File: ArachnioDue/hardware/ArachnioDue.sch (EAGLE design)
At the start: 55 parts, among them J6 HEAD17-NOSS, Q1 12MHz, U1 SAM3SB-AU, U2 AP2111HA-3.3

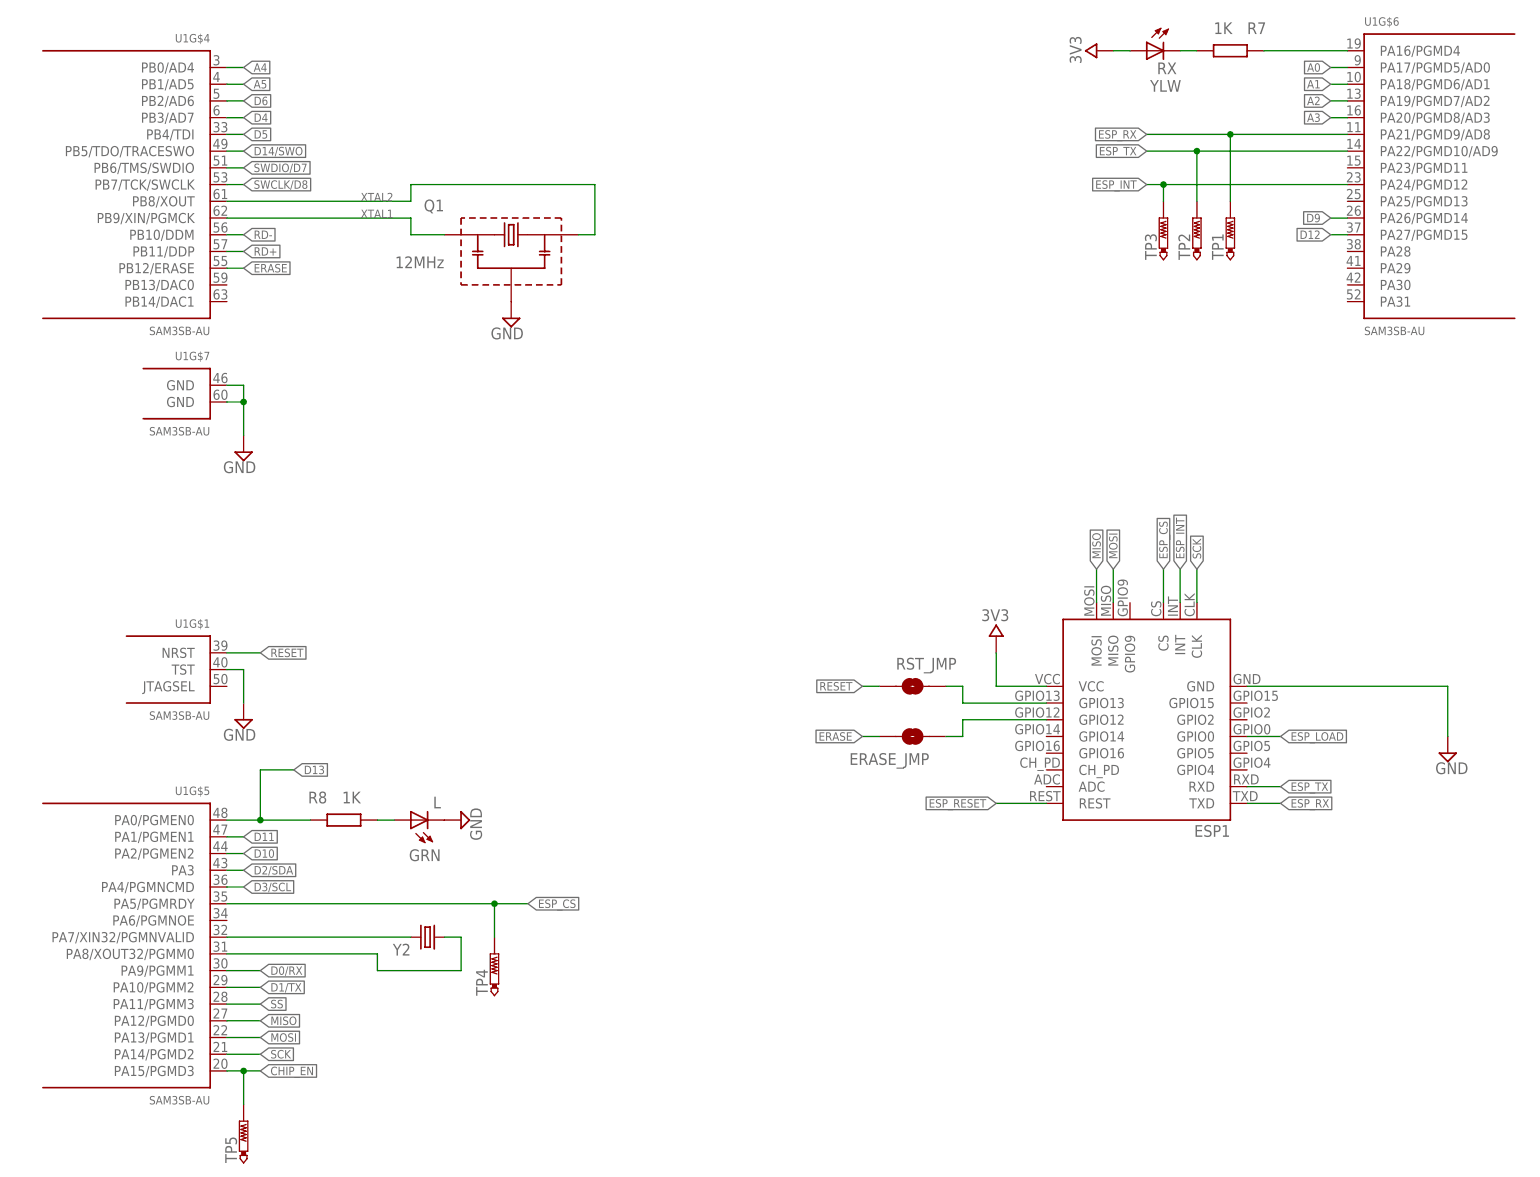
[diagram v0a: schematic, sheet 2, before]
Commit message: Some last changes to the schematic and layout
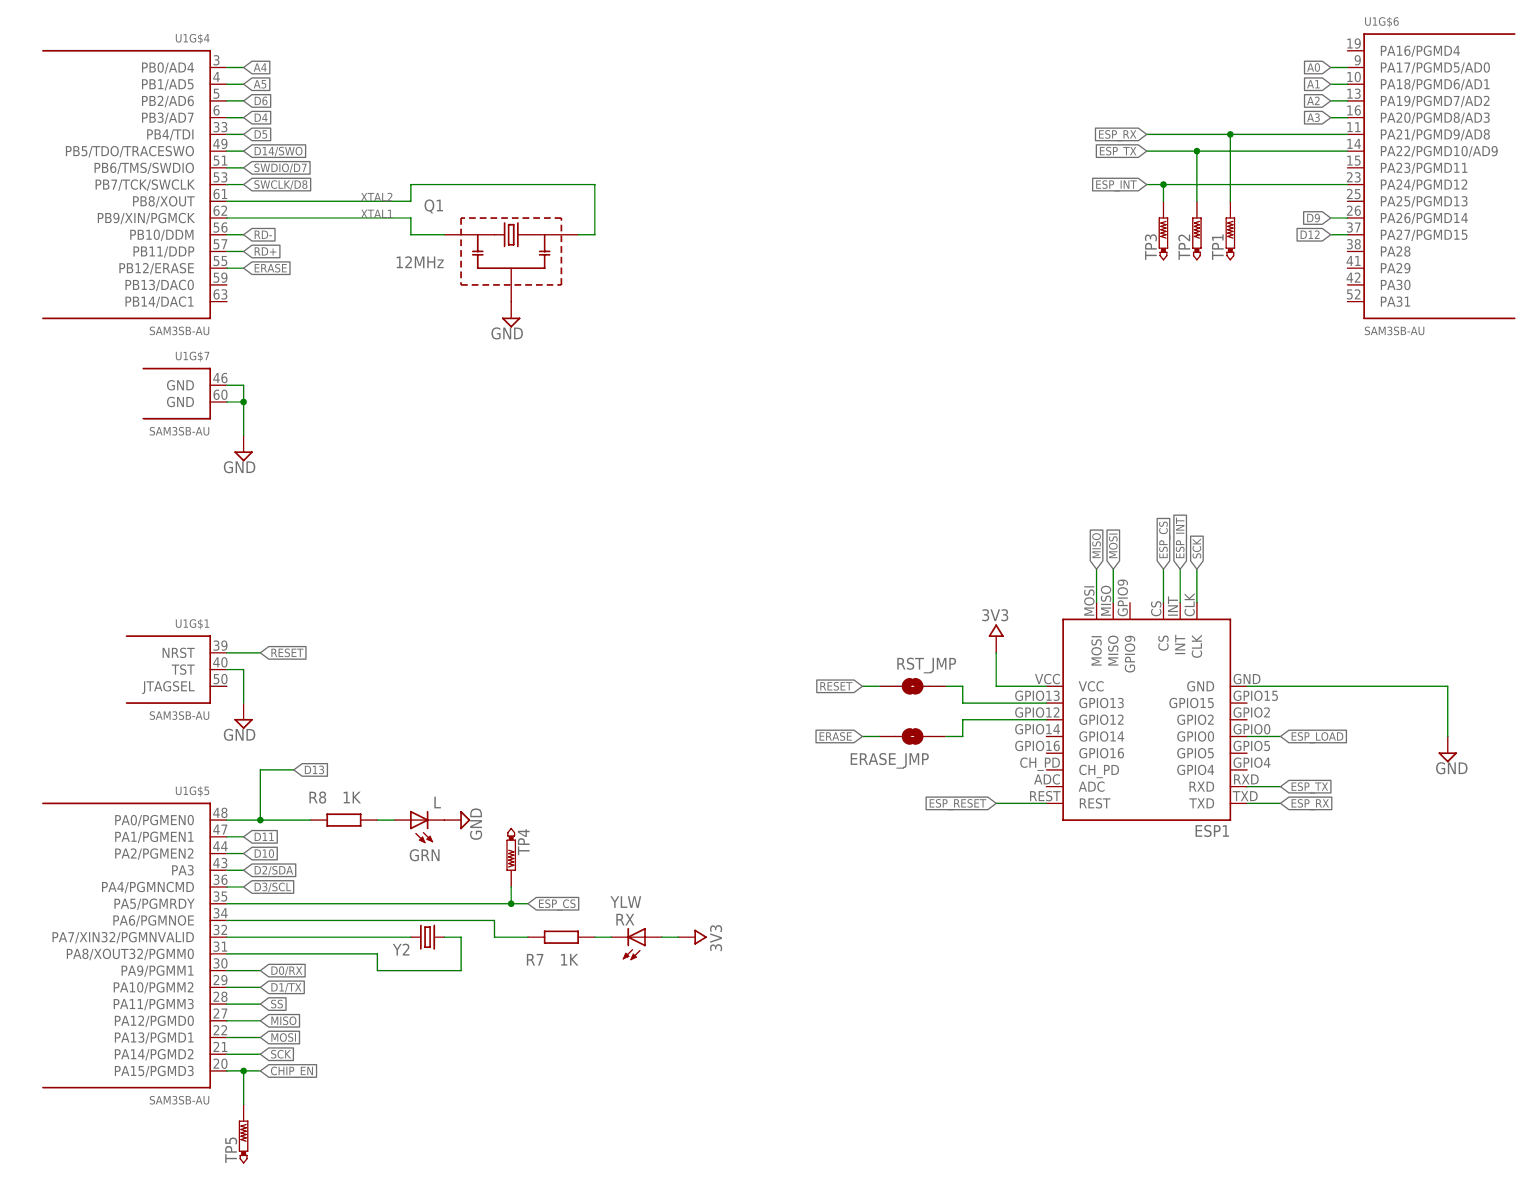
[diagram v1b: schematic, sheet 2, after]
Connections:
- net RXTXLED: now also U1G$5.PA6/PGMNOE; no longer U1G$6.PA16/PGMD4
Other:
- moved on the sheet: R7, RX, TP4
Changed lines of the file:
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@@
 <attribute name="PARTNO" x="88.9" y="73.66" size="1.778" layer="96" display="off"/>
 </instance>
-<instance part="RX" gate="G$1" x="200.66" y="190.5" smashed="yes" rot="MR270">
-<attribute name="NAME" x="205.232" y="186.944" size="1.778" layer="95" rot="MR0"/>
-<attribute name="VALUE" x="201.168" y="186.055" size="1.778" layer="96" rot="MR180"/>
-<attribute name="PARTNO" x="200.66" y="190.5" size="1.778" layer="96" rot="MR180" display="off"/>
-</instance>
-<instance part="R7" gate="G$1" x="213.36" y="190.5" smashed="yes" rot="R180">
-<attribute name="NAME" x="215.9" y="193.04" size="1.778" layer="95"/>
-<attribute name="VALUE" x="210.82" y="193.04" size="1.778" layer="96"/>
-<attribute name="PARTNO" x="213.36" y="190.5" size="1.778" layer="96" rot="MR0" display="off"/>
+<instance part="RX" gate="G$1" x="124.46" y="55.88" smashed="yes" rot="MR90">
+<attribute name="NAME" x="119.888" y="59.436" size="1.778" layer="95" rot="MR180"/>
+<attribute name="VALUE" x="123.952" y="60.325" size="1.778" layer="96" rot="MR0"/>
+<attribute name="PARTNO" x="124.46" y="55.88" size="1.778" layer="96" rot="MR0" display="off"/>
+</instance>
+<instance part="R7" gate="G$1" x="111.76" y="55.88" smashed="yes">
+<attribute name="NAME" x="109.22" y="53.34" size="1.778" layer="95" rot="R180"/>
+<attribute name="VALUE" x="114.3" y="53.34" size="1.778" layer="96" rot="R180"/>
+<attribute name="PARTNO" x="111.76" y="55.88" size="1.778" layer="96" rot="MR180" display="off"/>
 </instance>
 <instance part="R8" gate="G$1" x="78.74" y="73.66" smashed="yes" rot="MR180">
@@
 <attribute name="PARTNO" x="91.44" y="55.88" size="1.27" layer="96" display="off"/>
 </instance>
-<instance part="U$20" gate="G$1" x="193.04" y="190.5" rot="MR270"/>
+<instance part="U$20" gate="G$1" x="132.08" y="55.88" rot="MR90"/>
 <instance part="SUPPLY8" gate="GND" x="96.52" y="73.66" rot="MR270"/>
 <instance part="ESP1" gate="G$1" x="200.66" y="96.52" rot="MR180"/>
@@
 <instance part="TP2" gate="G$1" x="208.28" y="165.1"/>
 <instance part="TP3" gate="G$1" x="203.2" y="165.1"/>
-<instance part="TP4" gate="G$1" x="101.6" y="53.34"/>
+<instance part="TP4" gate="G$1" x="104.14" y="66.04" rot="R180"/>
 <instance part="TP5" gate="G$1" x="63.5" y="27.94"/>
 </instances>
@@
 <net name="RXTXLED" class="0">
 <segment>
+<pinref part="U1" gate="G$5" pin="PA6/PGMNOE"/>
+<wire x1="60.96" y1="58.42" x2="101.6" y2="58.42" width="0.1524" layer="91"/>
+<wire x1="101.6" y1="58.42" x2="101.6" y2="55.88" width="0.1524" layer="91"/>
 <pinref part="R7" gate="G$1" pin="1"/>
-<pinref part="U1" gate="G$6" pin="PA16/PGMD4"/>
-<wire x1="231.14" y1="190.5" x2="218.44" y2="190.5" width="0.1524" layer="91"/>
+<wire x1="101.6" y1="55.88" x2="106.68" y2="55.88" width="0.1524" layer="91"/>
 </segment>
 </net>
@@
 <pinref part="RX" gate="G$1" pin="A"/>
 <pinref part="U$20" gate="G$1" pin="3V3"/>
-<wire x1="198.12" y1="190.5" x2="195.58" y2="190.5" width="0.1524" layer="91"/>
+<wire x1="127" y1="55.88" x2="129.54" y2="55.88" width="0.1524" layer="91"/>
 </segment>
 <segment>
@@
 <pinref part="R7" gate="G$1" pin="2"/>
 <pinref part="RX" gate="G$1" pin="C"/>
-<wire x1="205.74" y1="190.5" x2="208.28" y2="190.5" width="0.1524" layer="91"/>
+<wire x1="119.38" y1="55.88" x2="116.84" y2="55.88" width="0.1524" layer="91"/>
 </segment>
 </net>
@@
 <segment>
 <pinref part="U1" gate="G$5" pin="PA5/PGMRDY"/>
-<wire x1="60.96" y1="60.96" x2="101.6" y2="60.96" width="0.1524" layer="91"/>
+<wire x1="60.96" y1="60.96" x2="104.14" y2="60.96" width="0.1524" layer="91"/>
 <label x="106.68" y="60.96" size="1.27" layer="95" xref="yes"/>
 <pinref part="TP4" gate="G$1" pin="TP"/>
-<wire x1="101.6" y1="60.96" x2="106.68" y2="60.96" width="0.1524" layer="91"/>
-<wire x1="101.6" y1="60.96" x2="101.6" y2="55.88" width="0.1524" layer="91"/>
-<junction x="101.6" y="60.96"/>
-</segment>
-</net>
+<wire x1="104.14" y1="60.96" x2="106.68" y2="60.96" width="0.1524" layer="91"/>
+<wire x1="104.14" y1="60.96" x2="104.14" y2="63.5" width="0.1524" layer="91"/>
+<junction x="104.14" y="60.96"/>
+</segment>
+</net>
